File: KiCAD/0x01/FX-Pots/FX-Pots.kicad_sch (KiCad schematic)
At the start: 28 parts, among them J1 Conn_01x05, J2 Conn_01x05, SW1 SW_Push_LED, SW2 SW_Push_LED, SW3 SW_Push_LED, SW4 SW_Push_LED, U1 74HC595, U2 CD74HC4067M

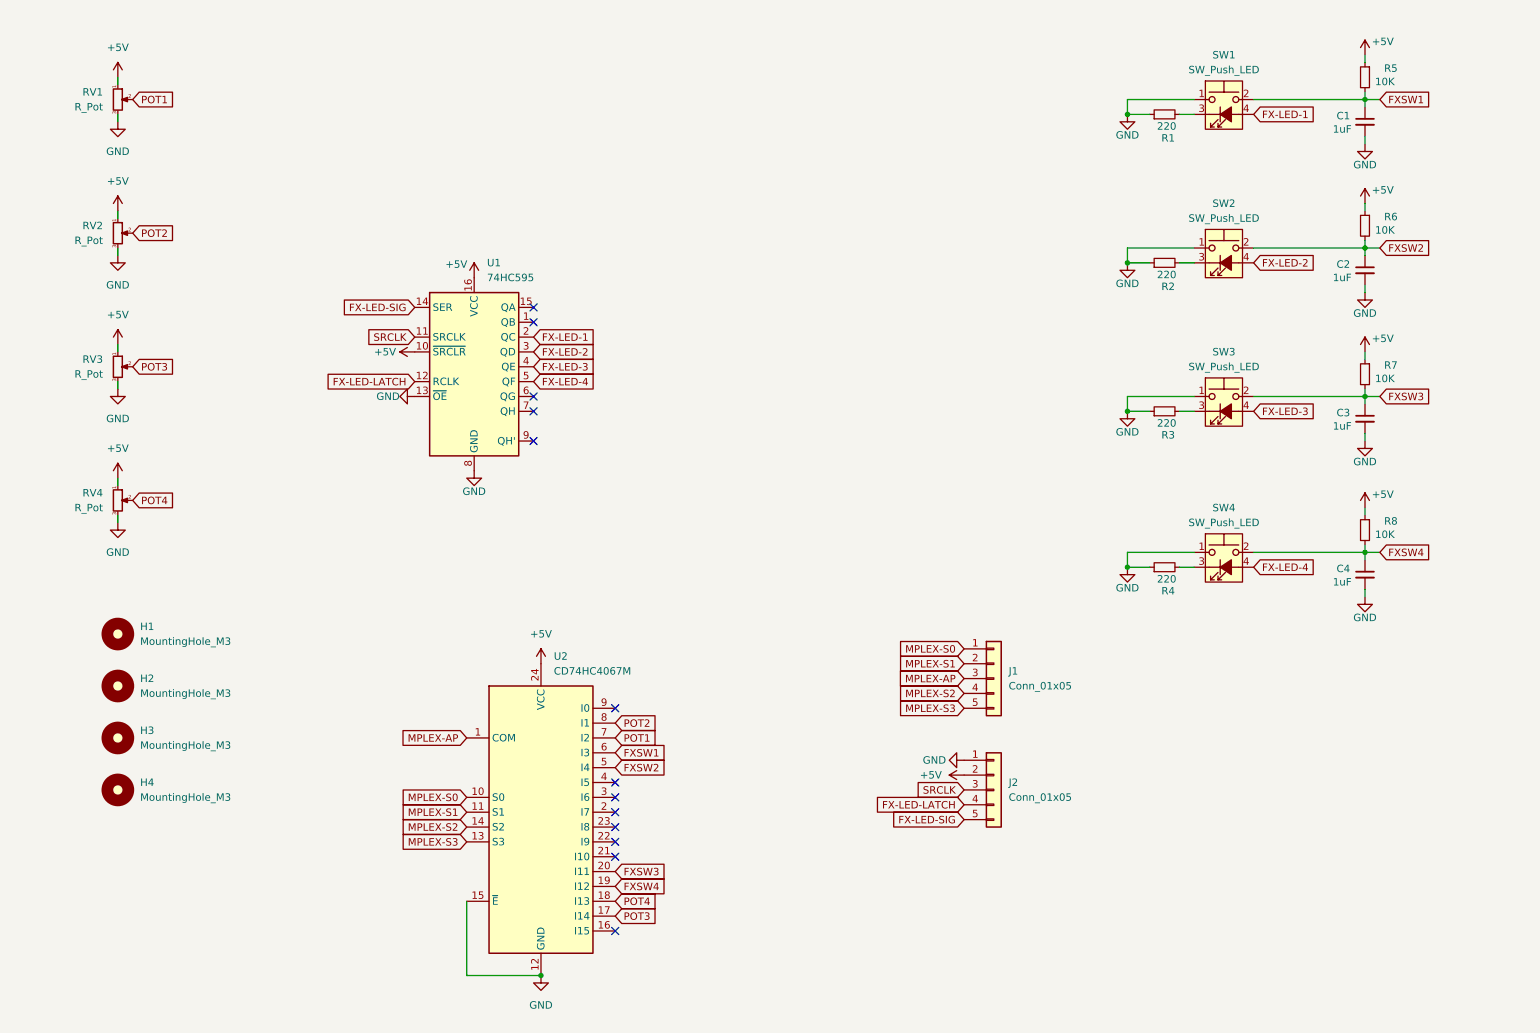
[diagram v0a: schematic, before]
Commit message: fx-pots
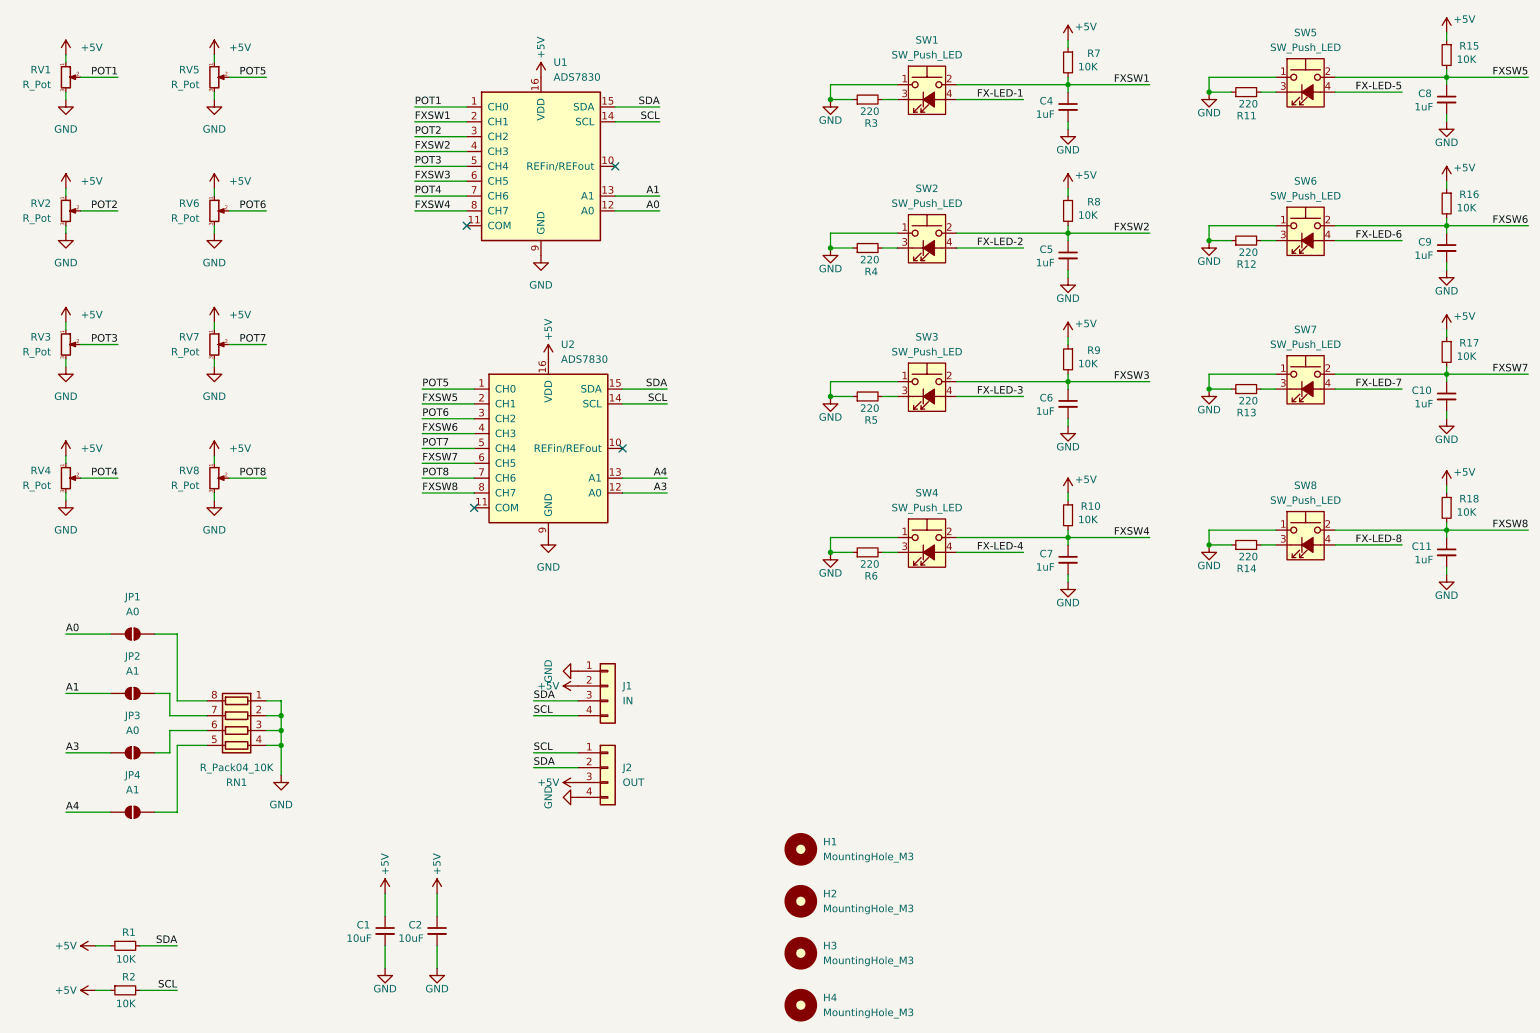
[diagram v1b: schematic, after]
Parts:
- removed J1, J2: Conn_01x05, Connector_PinSocket_2.54mm:PinSocket_1x05_P2.54mm_Vertical, symbol Connector_Generic:Conn_01x05
- removed U1: 74HC595, Package_SO:SOIC-16_3.9x9.9mm_P1.27mm, symbol 74xx:74HC595
- removed U2: CD74HC4067M, Package_SO:SOIC-24W_7.5x15.4mm_P1.27mm, symbol 74xx:CD74HC4067M
- added C1, C2: 10uF, Capacitor_SMD:C_0805_2012Metric_Pad1.18x1.45mm_HandSolder, symbol Device:C_Small
- added C10, C11, C8, C9: 1uF, Capacitor_SMD:C_1206_3216Metric_Pad1.33x1.80mm_HandSolder, symbol Device:C_Small
- added J1: IN, Connector_JST:JST_PH_S4B-PH-K_1x04_P2.00mm_Horizontal, symbol Connector_Generic:Conn_01x04
- added J2: OUT, Connector_JST:JST_PH_S4B-PH-K_1x04_P2.00mm_Horizontal, symbol Connector_Generic:Conn_01x04
- added JP1, JP3: A0, Jumper:SolderJumper-2_P1.3mm_Open_RoundedPad1.0x1.5mm, symbol Jumper:SolderJumper_2_Open
- added JP2, JP4: A1, Jumper:SolderJumper-2_P1.3mm_Open_RoundedPad1.0x1.5mm, symbol Jumper:SolderJumper_2_Open
- added R1, R2: 10K, Capacitor_SMD:C_0805_2012Metric_Pad1.18x1.45mm_HandSolder, symbol Device:R_Small
- added R11, R12, R13, R14: 220, PCM_Resistor_SMD_AKL:R_1206_3216Metric_Pad1.30x1.75mm_HandSolder, symbol Device:R_Small
- added R15, R16, R17, R18: 10K, PCM_Resistor_SMD_AKL:R_1206_3216Metric_Pad1.30x1.75mm_HandSolder, symbol Device:R_Small
- added RN1: R_Pack04_10K, Resistor_SMD:R_Array_Convex_4x0603, symbol Device:R_Pack04
- added RV5, RV6, RV7, RV8: R_Pot, Potentiometer_THT:Potentiometer_Bourns_PTV09A-1_Single_Vertical, symbol Device:R_Potentiometer_Small
- added SW5, SW6, SW7, SW8: SW_Push_LED, led-switch:SW_PUSH_6mm_LED, symbol Switch:SW_Push_LED
- added U1, U2: ADS7830, Package_SO:TSSOP-16_4.4x5mm_P0.65mm, symbol Analog_DAC:ADS7830
- SW1, SW2, SW3, SW4: footprint led-sw:led switch -> led-switch:SW_PUSH_6mm_LED
- renumbered C1 to C4, C2 to C5, C3 to C6, C4 to C7, R8 to R10, R1 to R3, R2 to R4, R3 to R5, R4 to R6, R5 to R7, R6 to R8, R7 to R9
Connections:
- net +5V: now also C1.1, C2.1, J1.2 (Pin_2), J2.3 (Pin_3), R1.1, R15.1, R16.1, R17.1, R18.1, R2.1, RV5.1, RV6.1, RV7.1, RV8.1, U1.16 (VDD), U2.16 (VDD)
- net FXSW1: now also U1.2 (CH1)
- net FXSW2: now also U1.4 (CH3)
- net FXSW3: now also U1.6 (CH5)
- net FXSW4: now also U1.8 (CH7)
- net GND: now also C1.2, C10.2, C11.2, C2.2, C8.2, C9.2, J1.1 (Pin_1), J2.4 (Pin_4), R11.1, R12.1, R13.1, R14.1, RN1.1 (R1.1), RN1.2 (R2.1), RN1.3 (R3.1), RN1.4 (R4.1), RV5.3, RV6.3, RV7.3, RV8.3, SW5.1, SW6.1, SW7.1, SW8.1, U1.9 (GND), U2.9 (GND)
- net POT1: now also U1.1 (CH0)
- net POT2: now also U1.3 (CH2)
- net POT3: now also U1.5 (CH4)
- net POT4: now also U1.7 (CH6)
- new net: R14.2, SW8.3 (K)
- new net: R12.2, SW6.3 (K)
- new net: R13.2, SW7.3 (K)
- new net: JP4.2 (B), RN1.5 (R4.2)
- new net: JP2.2 (B), RN1.7 (R2.2)
- new net: R11.2, SW5.3 (K)
- new net: JP3.2 (B), RN1.6 (R3.2)
- new net: JP1.2 (B), RN1.8 (R1.2)
- new net A0: JP1.1 (A), U1.12 (A0)
- new net A1: JP2.1 (A), U1.13 (A1)
- new net A3: JP3.1 (A), U2.12 (A0)
- new net A4: JP4.1 (A), U2.13 (A1)
- new net FX-LED-5: SW5.4 (A)
- new net FX-LED-6: SW6.4 (A)
- new net FX-LED-7: SW7.4 (A)
- new net FX-LED-8: SW8.4 (A)
- new net FXSW5: C8.1, R15.2, SW5.2, U2.2 (CH1)
- new net FXSW6: C9.1, R16.2, SW6.2, U2.4 (CH3)
- new net FXSW7: C10.1, R17.2, SW7.2, U2.6 (CH5)
- new net FXSW8: C11.1, R18.2, SW8.2, U2.8 (CH7)
- new net POT5: RV5.2, U2.1 (CH0)
- new net POT6: RV6.2, U2.3 (CH2)
- new net POT7: RV7.2, U2.5 (CH4)
- new net POT8: RV8.2, U2.7 (CH6)
- new net SCL: J1.4 (Pin_4), J2.1 (Pin_1), R2.2, U1.14 (SCL), U2.14 (SCL)
- new net SDA: J1.3 (Pin_3), J2.2 (Pin_2), R1.2, U1.15 (SDA), U2.15 (SDA)
- no-connect marks 13 -> 4
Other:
- moved on the sheet: C4, C5, C6, C7, H1, H2, H3, H4, R10, R3, R4, R5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
